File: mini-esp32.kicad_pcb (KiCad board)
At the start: 4 copper layers, 29 x 58 mm, 46 parts, among them J1 BAT, J2 USB_B_Micro, J5 Conn_01x18, J6 Conn_01x18, Q1 AO3401A, Q2 S8050, Q3 S8050, Q4 2N7002, SW1 RESET, U1 ESP32-WROOM-32D, U2 RT9080-33GJ5, U3 TP4056, U4 CH340G, Y1 12MHz

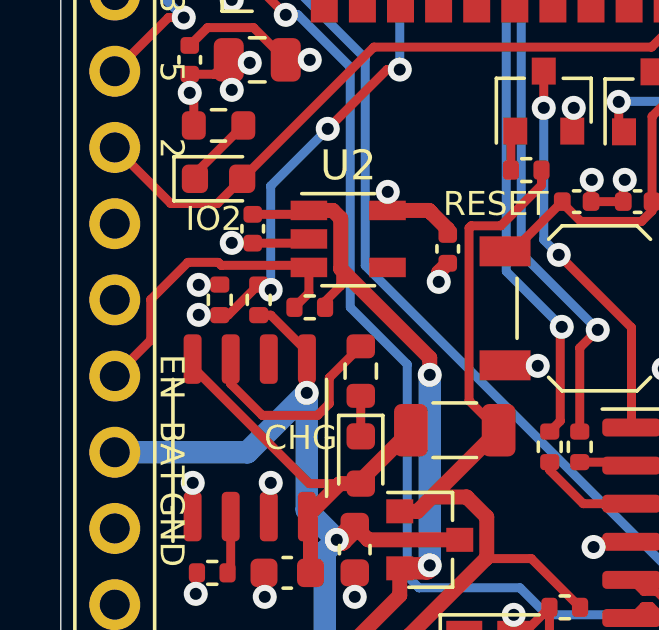
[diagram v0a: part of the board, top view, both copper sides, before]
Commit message: Rename files
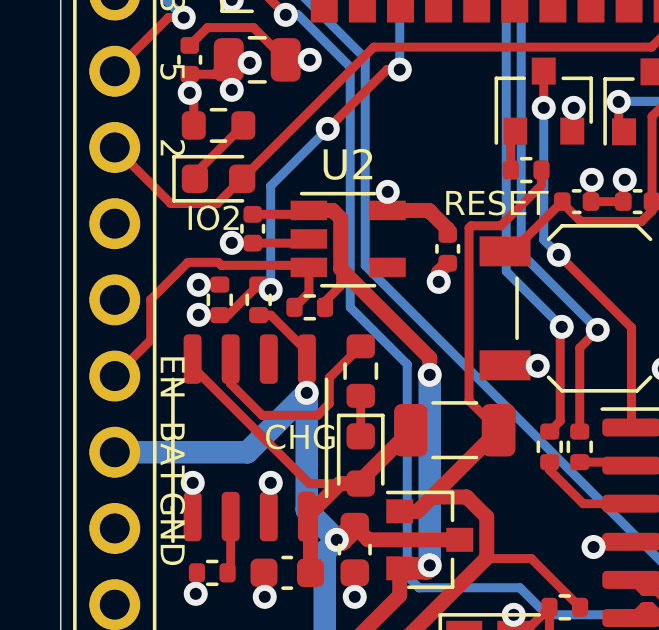
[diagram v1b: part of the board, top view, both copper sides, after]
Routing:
- net I35: track 44.7 -> 45.4 mm
